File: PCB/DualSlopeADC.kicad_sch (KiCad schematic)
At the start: 18 parts, among them J1 RPi_GPIO, J5 Conn_01x02, J6 Conn_01x02, J7 Conn_01x02, Q1 PMOS, Q2 NMOS, Q4 PNP, U1 OPA1692xDGK, U2 OPA1692xDGK, U3 OPA1692xDGK

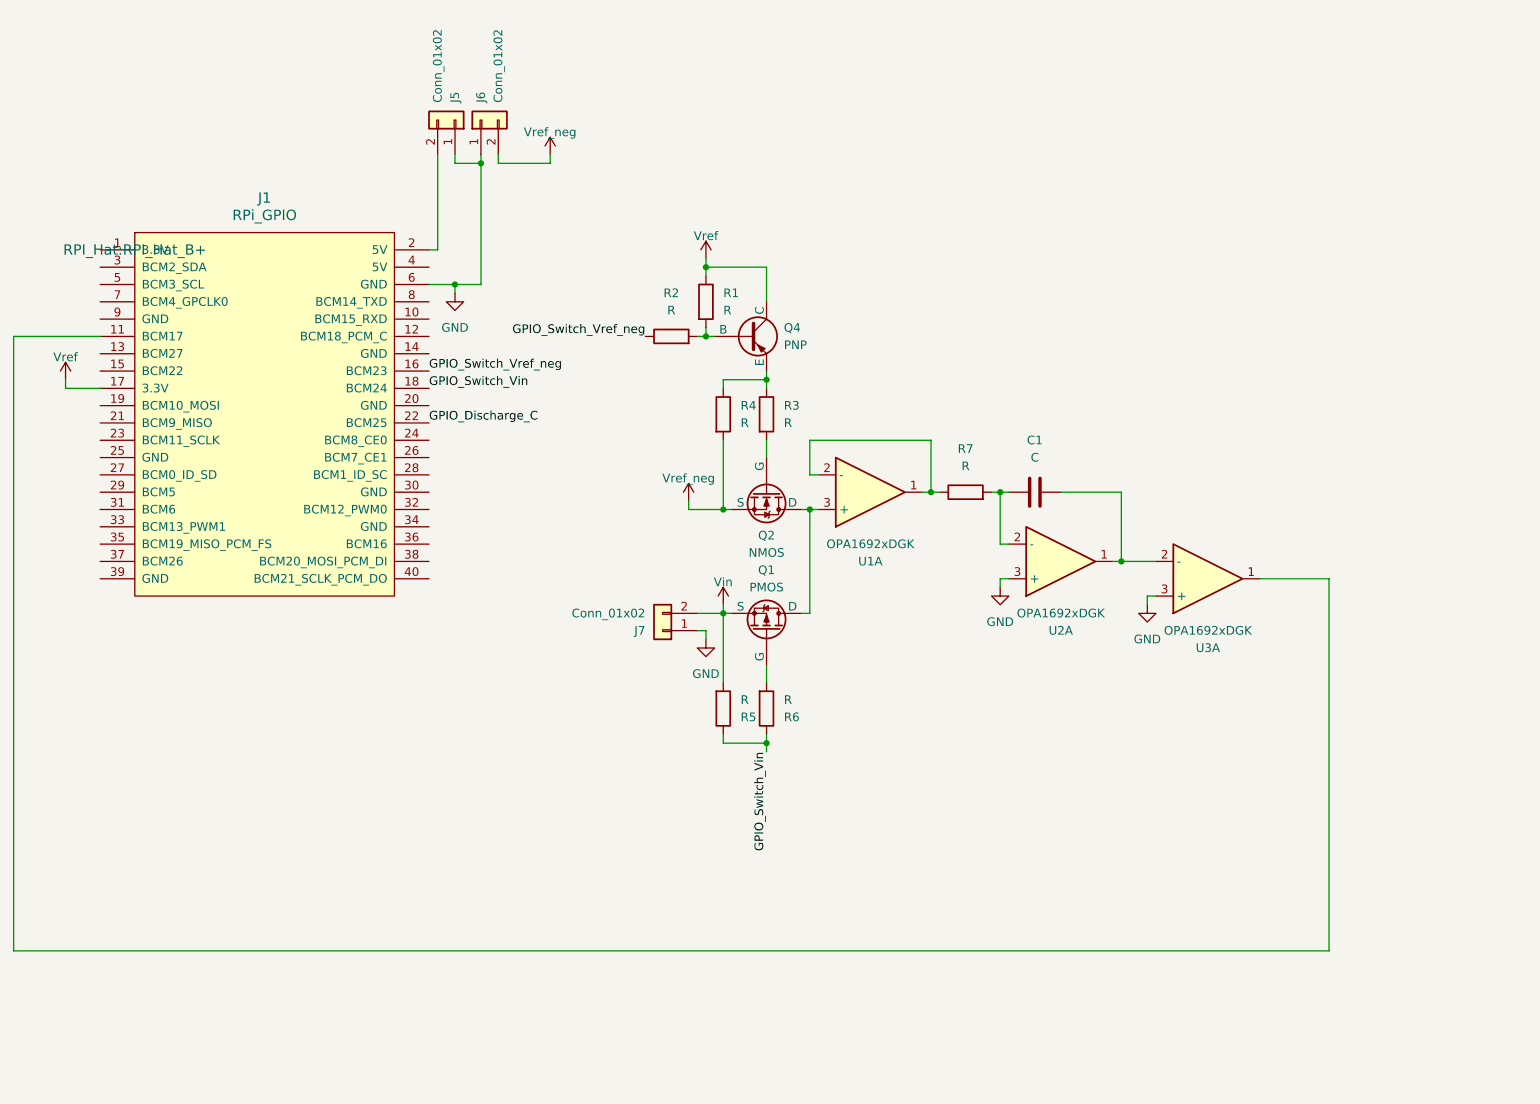
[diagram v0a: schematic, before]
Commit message: .
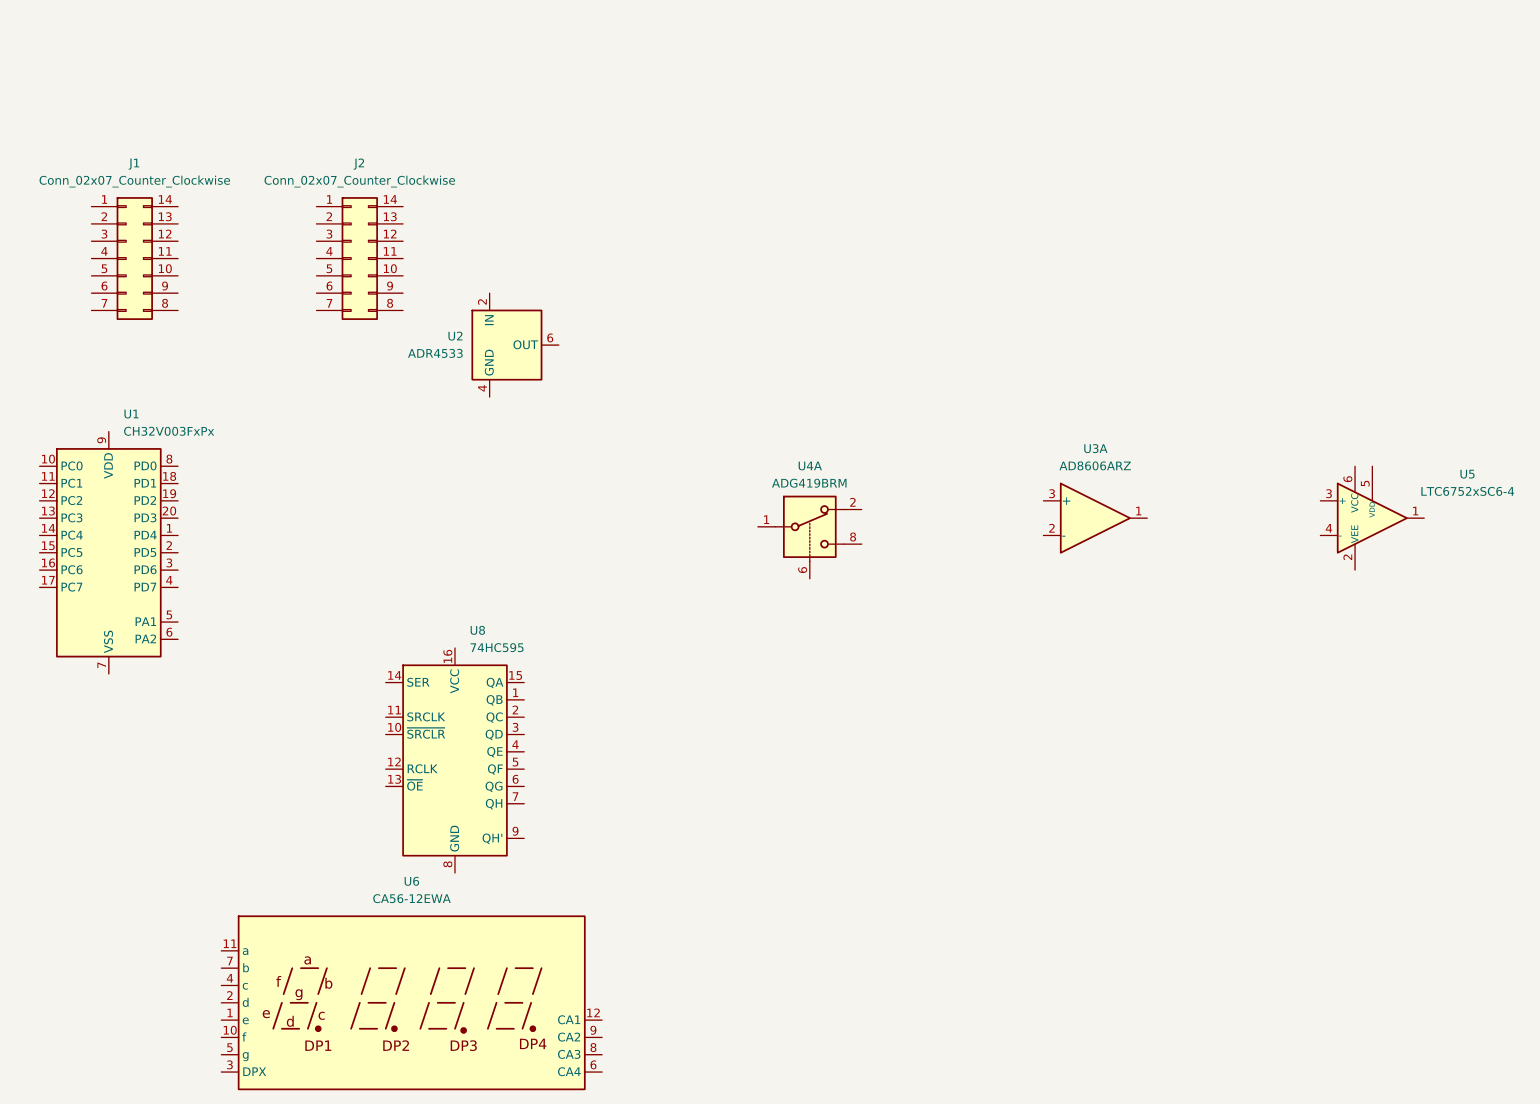
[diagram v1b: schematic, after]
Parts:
- removed C1: C, Capacitor_SMD:C_0805_2012Metric, symbol Device:C
- removed J1: RPi_GPIO, RPI_Hat:RPI_Hat_B+, symbol RPi_Hat:RPi_GPIO
- removed J5, J6, J7: Conn_01x02, Connector_PinHeader_2.54mm:PinHeader_1x02_P2.54mm_Vertical, symbol Connector_Generic:Conn_01x02
- removed Q1: PMOS, symbol Simulation_SPICE:PMOS
- removed Q2: NMOS, symbol Simulation_SPICE:NMOS
- removed Q4: PNP, symbol Simulation_SPICE:PNP
- removed R1, R2, R3, R4, R5, R6, R7: R, Resistor_SMD:R_0603_1608Metric, symbol Device:R
- removed U1, U2, U3: OPA1692xDGK, Package_SO:VSSOP-8_3x3mm_P0.65mm, symbol Amplifier_Operational:OPA1692xDGK
- added J1, J2: Conn_02x07_Counter_Clockwise, Connector_PinHeader_2.54mm:PinHeader_2x07_P2.54mm_Vertical, symbol Connector_Generic:Conn_02x07_Counter_Clockwise
- added U1: CH32V003FxPx, Package_SO:TSSOP-20_4.4x6.5mm_P0.65mm, symbol MCU_WCH_CH32V0:CH32V003FxPx
- added U2: ADR4533, Package_SO:SOIC-8_3.9x4.9mm_P1.27mm, symbol Reference_Voltage:ADR4533
- added U3: AD8606ARZ, Package_SO:SOIC-8_3.9x4.9mm_P1.27mm, symbol Amplifier_Operational:AD8606ARZ
- added U4: ADG419BRM, Package_SO:MSOP-8_3x3mm_P0.65mm, symbol Analog_Switch:ADG419BRM
- added U5: LTC6752xSC6-4, Package_TO_SOT_SMD:SOT-363_SC-70-6, symbol Comparator:LTC6752xSC6-4
- added U6: CA56-12EWA, Display_7Segment:CA56-12EWA, symbol Display_Character:CA56-12EWA
- added U8: 74HC595, Package_DIP:DIP-16_W7.62mm, symbol 74xx:74HC595
